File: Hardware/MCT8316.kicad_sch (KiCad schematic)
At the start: 32 parts, among them J5 Screw_Terminal_01x03, J6 Screw_Terminal_01x03, J7 Conn_01x04_Male, J8 Conn_01x03_Pin, U10 MCT8316, U12 ISO7721DR

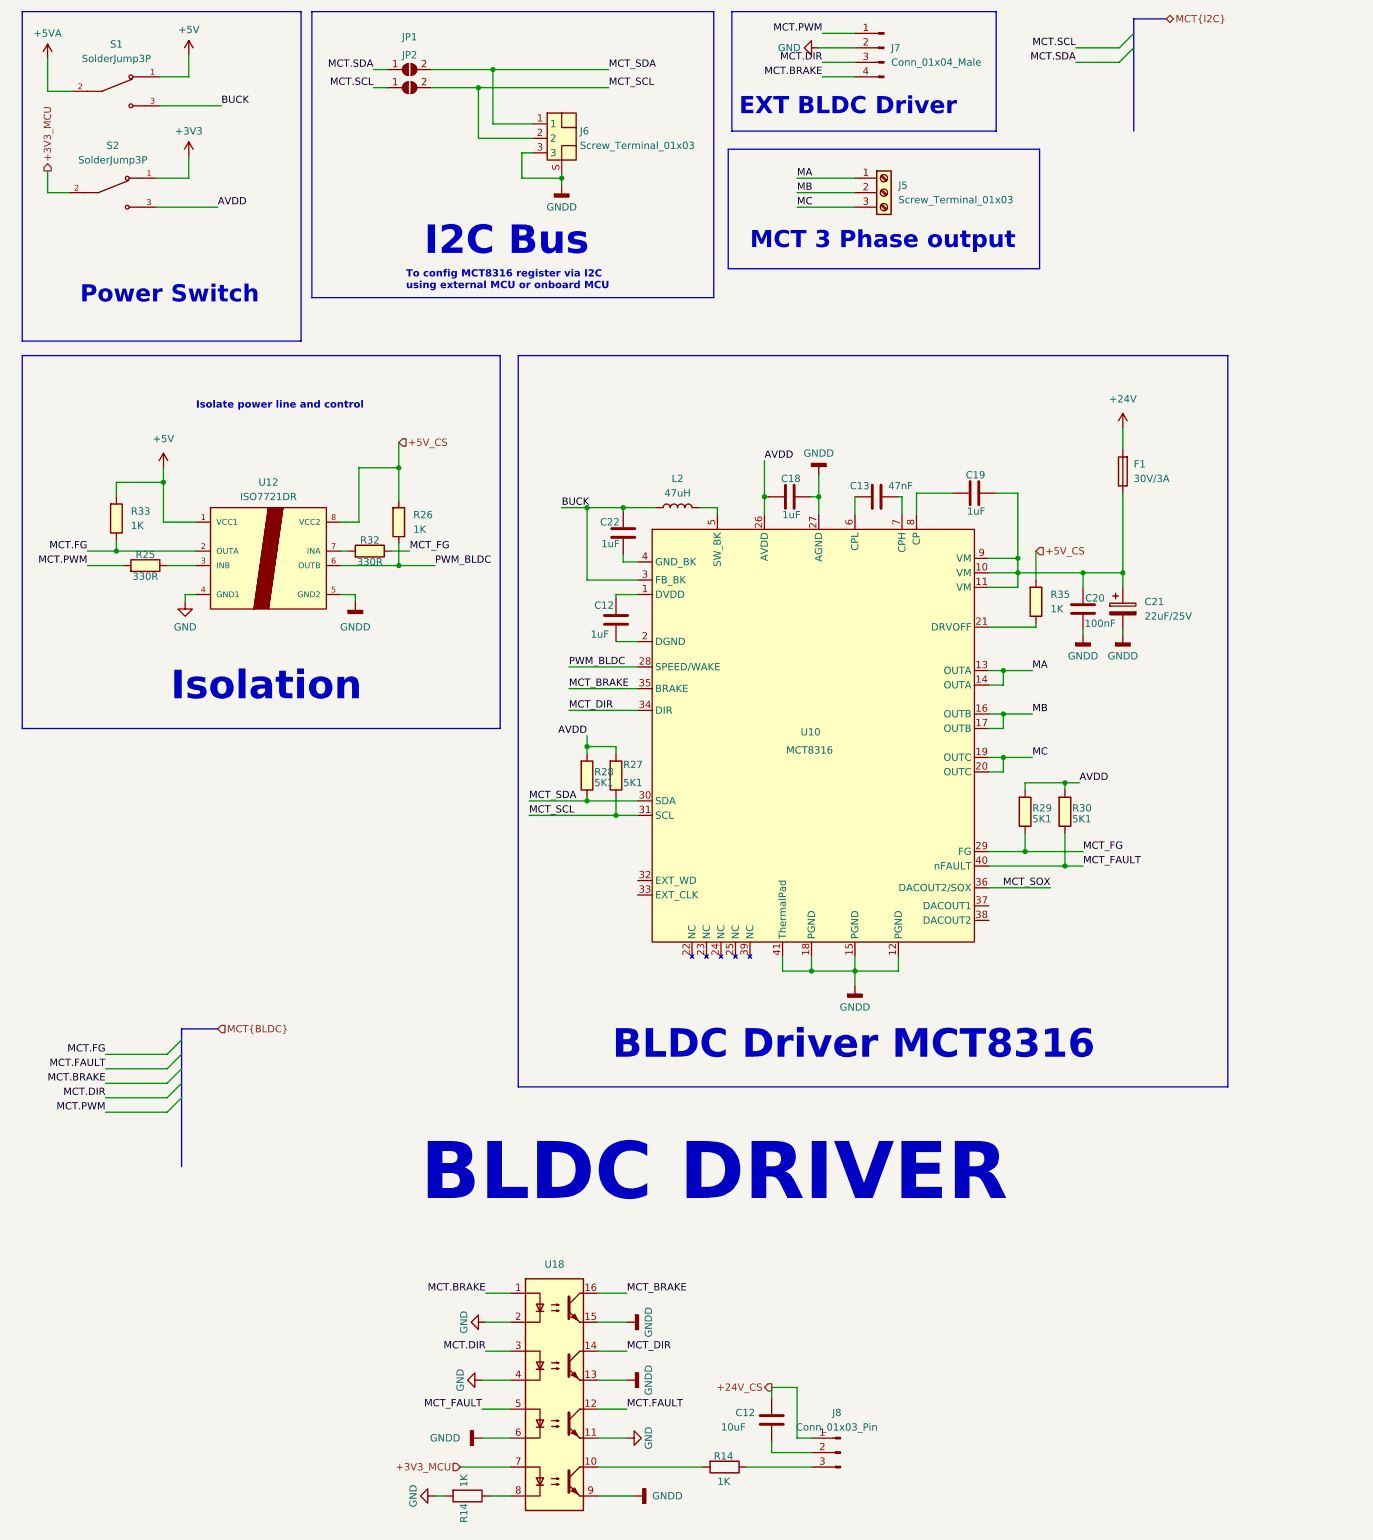
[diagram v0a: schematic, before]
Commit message: Fix bug schematic
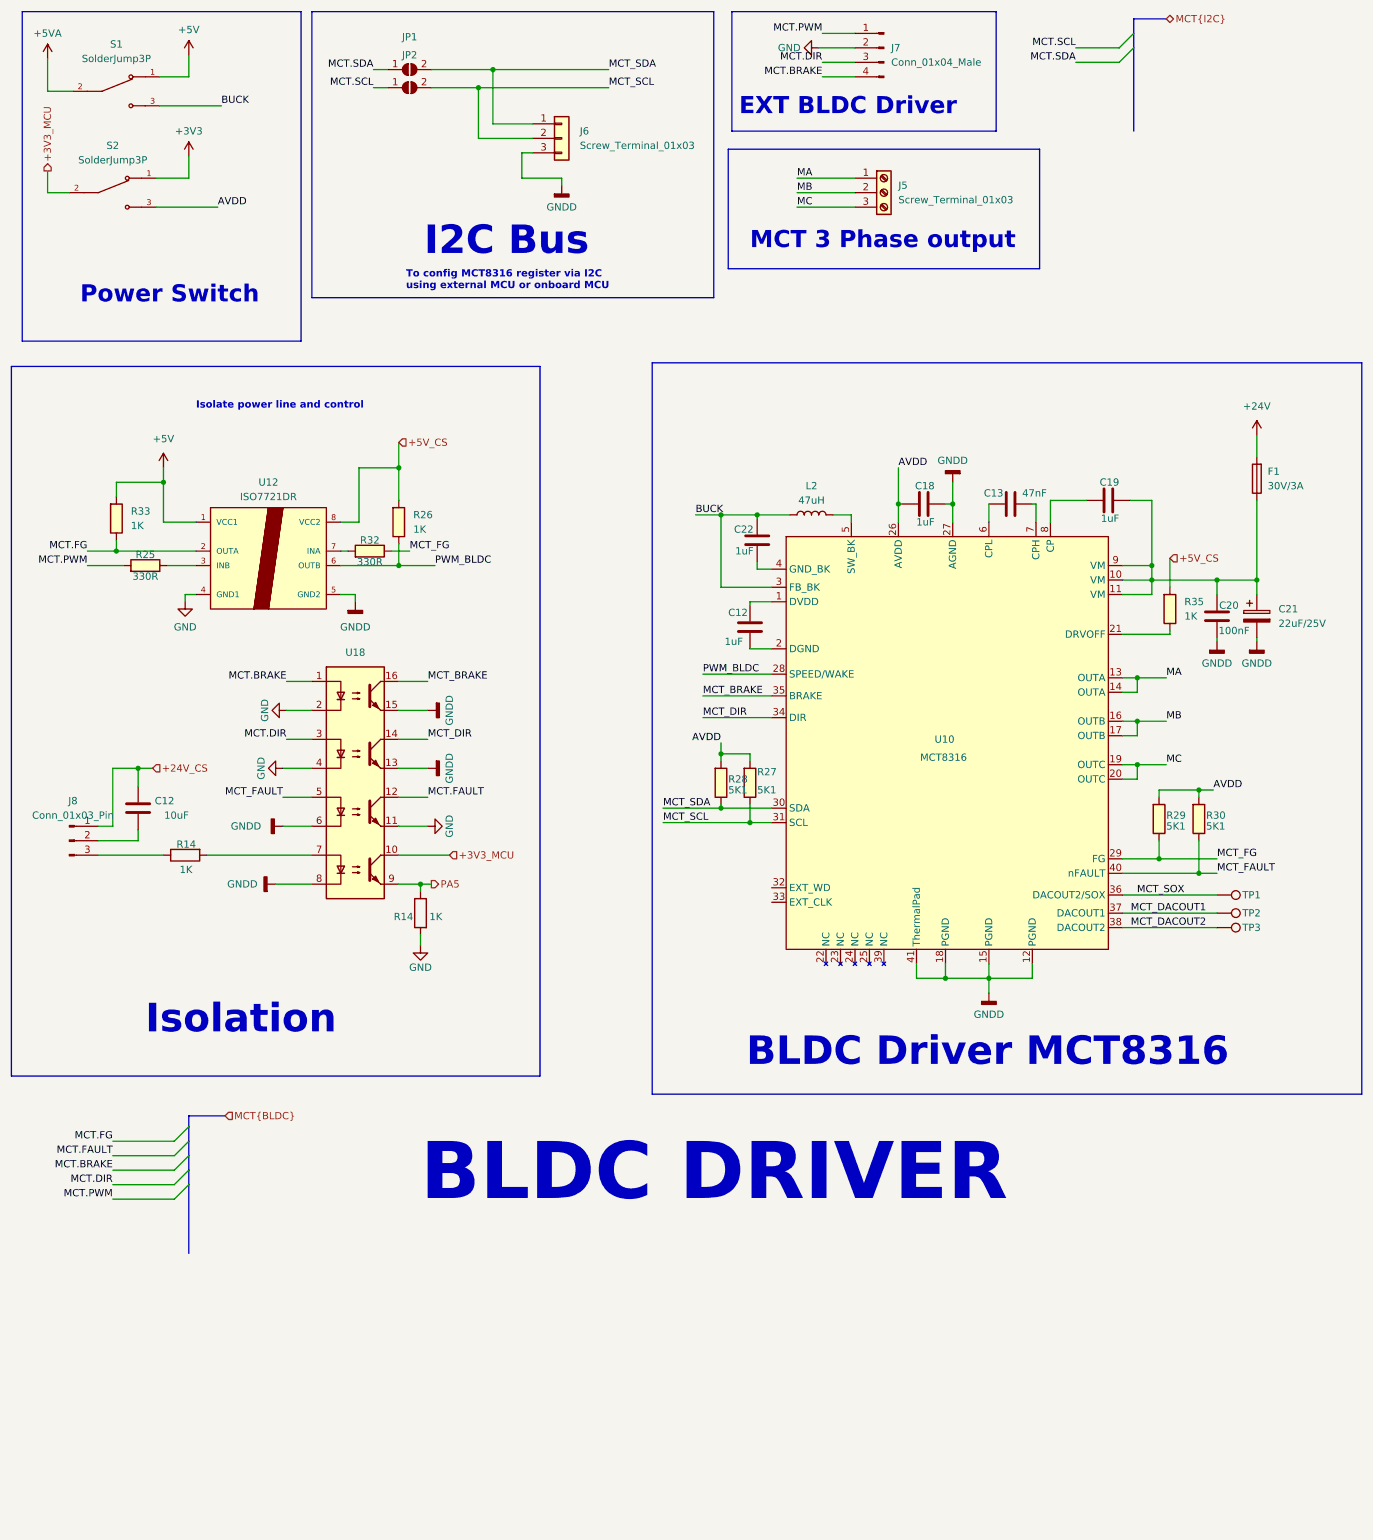
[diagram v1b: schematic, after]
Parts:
- added TP1, TP2, TP3: TestPoint, IVS_FOOTPRINTS:TestPoint_Pad_D1.0mm, symbol IVS_SYMBOLS:TestPoint
- C12, C18, C19, C22: footprint IVS_FOOTPRINTS:C_0603 -> IVS_FOOTPRINTS:C_0805
- J6: footprint IVS_FOOTPRINTS:Conn-Horz-SMD-3P-2.54mm-S3B_XH_SM4_TB -> IVS_FOOTPRINTS:XH_3P_2.54mm_Vertical; symbol IVS_SYMBOLS:Conn_JST_SMD_3P -> IVS_SYMBOLS:Conn_01x03
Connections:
- net +3V3_MCU: now also U18.10; no longer U18.7
- net GNDD: now also U18.8; no longer J6.S, U18.9
- net MCT_SOX: now also TP1.1
- net MCT_DACOUT1: now reaches U10.37 (DACOUT1)
- net MCT_DACOUT1: now also TP2.1
- net MCT_DACOUT2: now reaches U10.38 (DACOUT2)
- net MCT_DACOUT2: now also TP3.1
- net PA5: now reaches R14.1
- net PA5: now also U18.9; no longer U18.8
- net at R14.2: now also U18.7; no longer U18.10
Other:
- moved on the sheet: C12, C13, C18, C19, C20, C21, C22, F1, J8, L2, R14, R27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

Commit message: Voltage divider and Update I2C PinHeader
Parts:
- J6: footprint IVS_FOOTPRINTS:XH_3P_2.54mm_Vertical -> Connector_PinHeader_2.54mm:PinHeader_1x03_P2.54mm_Vertical
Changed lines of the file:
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@@
       (effects (font (size 1.27 1.27)) (justify left))
     )
-    (property "Footprint" "IVS_FOOTPRINTS:XH_3P_2.54mm_Vertical" (at 113.03 38.735 0)
+    (property "Footprint" "Connector_PinHeader_2.54mm:PinHeader_1x03_P2.54mm_Vertical" (at 113.03 38.735 0)
       (effects (font (size 1.27 1.27)) hide)
     )
